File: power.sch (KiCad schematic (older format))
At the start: 0 parts

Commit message: update,
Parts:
- added R?: R0, symbol taobao-r:R0
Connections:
- new net +3V3: R?.2
- new net Vrtc: R?.1

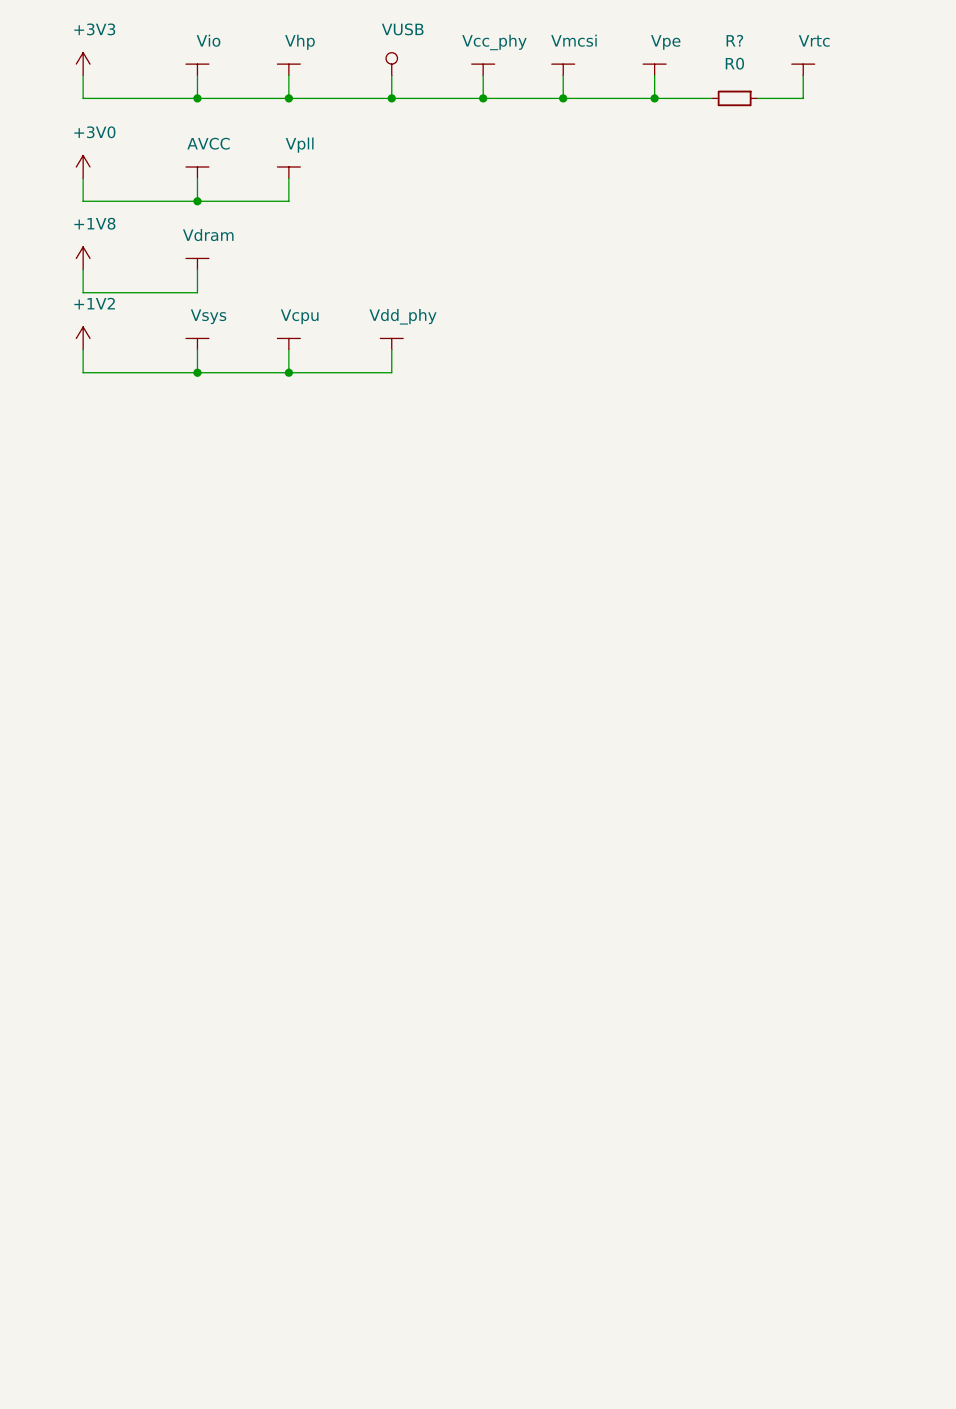
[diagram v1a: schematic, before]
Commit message: update,
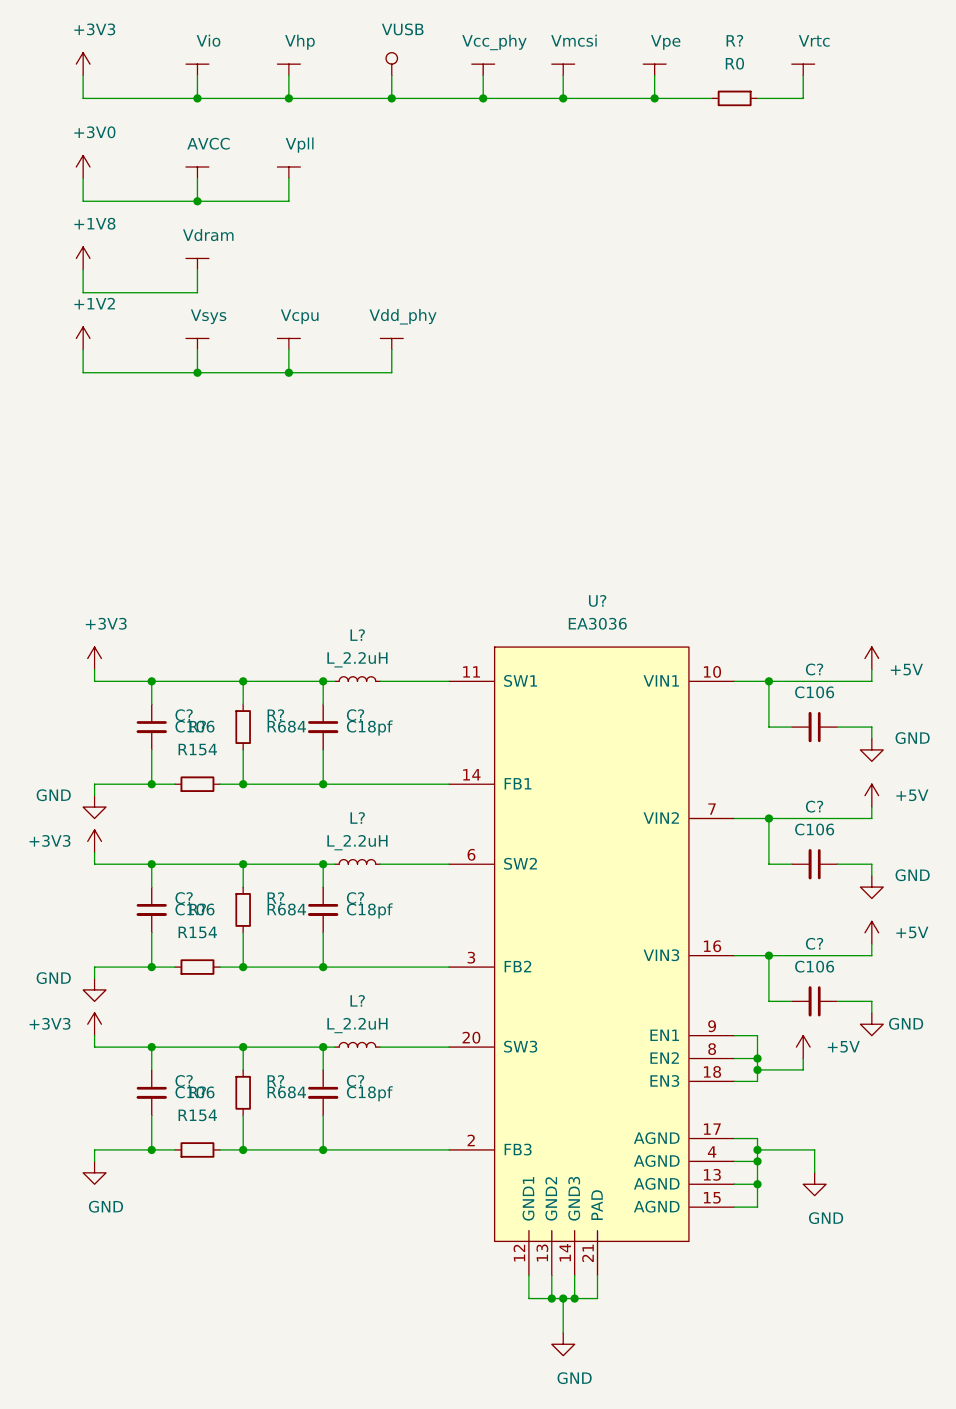
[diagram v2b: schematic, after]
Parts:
- added C? (x6): C106, symbol taobao-c:C106
- added C? (x3): C18pf, symbol taobao-c:C18pf
- added L? (x3): L_2.2uH, symbol taobao-l:L_2.2uH
- added R? (x3): R684, symbol taobao-r:R684
- added R? (x3): R154, symbol taobao-r:R154
- added U?: EA3036, symbol taobao-components:EA3036
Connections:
- net +3V3: now also C?.1, C?.1, C?.1, C?.1, C?.1, C?.1, L?.1, L?.1, L?.1, R?.1, R?.1, R?.1
- new net: L?.2, U?.11 (SW1)
- new net: C?.2, R?.2, R?.2, U?.14 (GND3)
- new net: C?.2, R?.2, R?.2, U?.2 (FB3)
- new net: L?.2, U?.20 (SW3)
- new net: C?.2, R?.2, R?.2, U?.3 (FB2)
- new net: L?.2, U?.6 (SW2)
- new net +5V: C?.2, C?.2, C?.2, U?.10 (VIN1), U?.16 (VIN3), U?.18 (EN3), U?.7 (VIN2), U?.8 (EN2), U?.9 (EN1)
- new net GND: C?.1, C?.1, C?.1, C?.2, C?.2, C?.2, R?.1, R?.1, R?.1, U?.12 (GND1), U?.13 (GND2), U?.14 (GND3), U?.15 (AGND), U?.17 (AGND), U?.21 (PAD), U?.4 (AGND)
